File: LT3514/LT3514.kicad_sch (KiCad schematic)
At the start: 15 parts, among them U1 LT3514xUFD

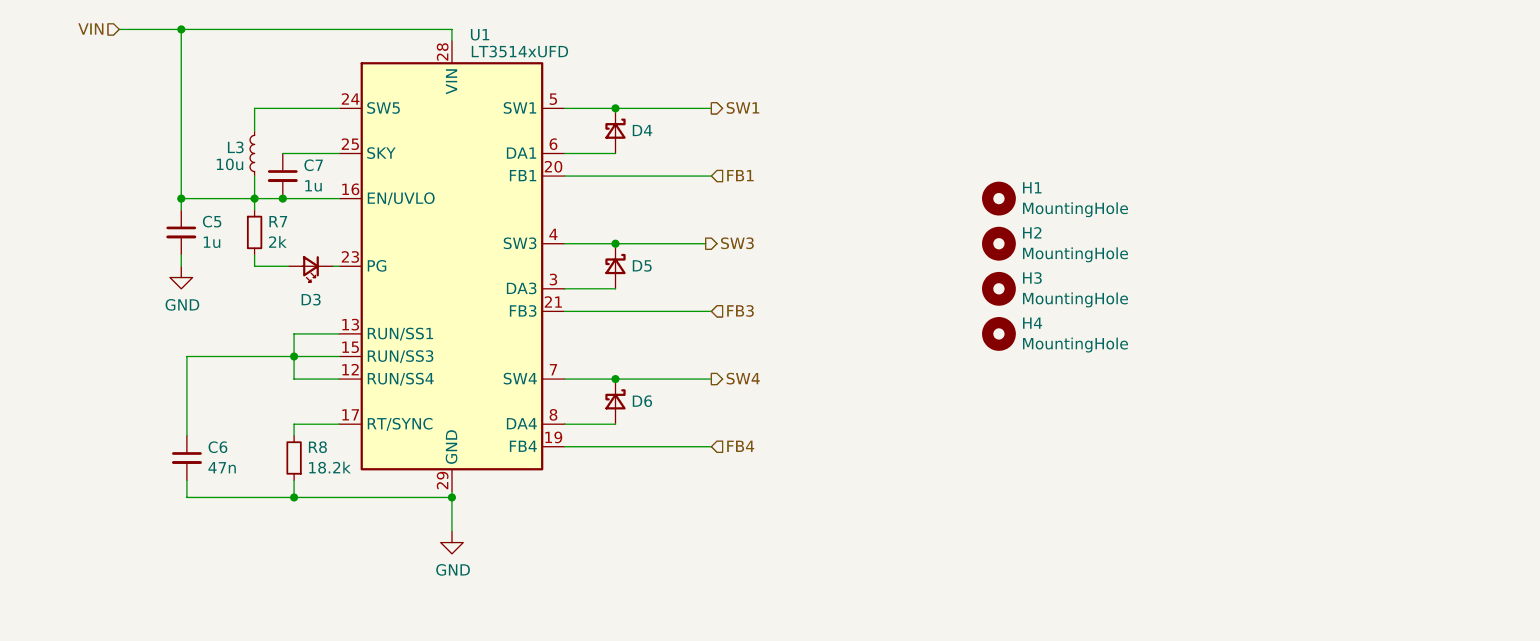
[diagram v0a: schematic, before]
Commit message: update files
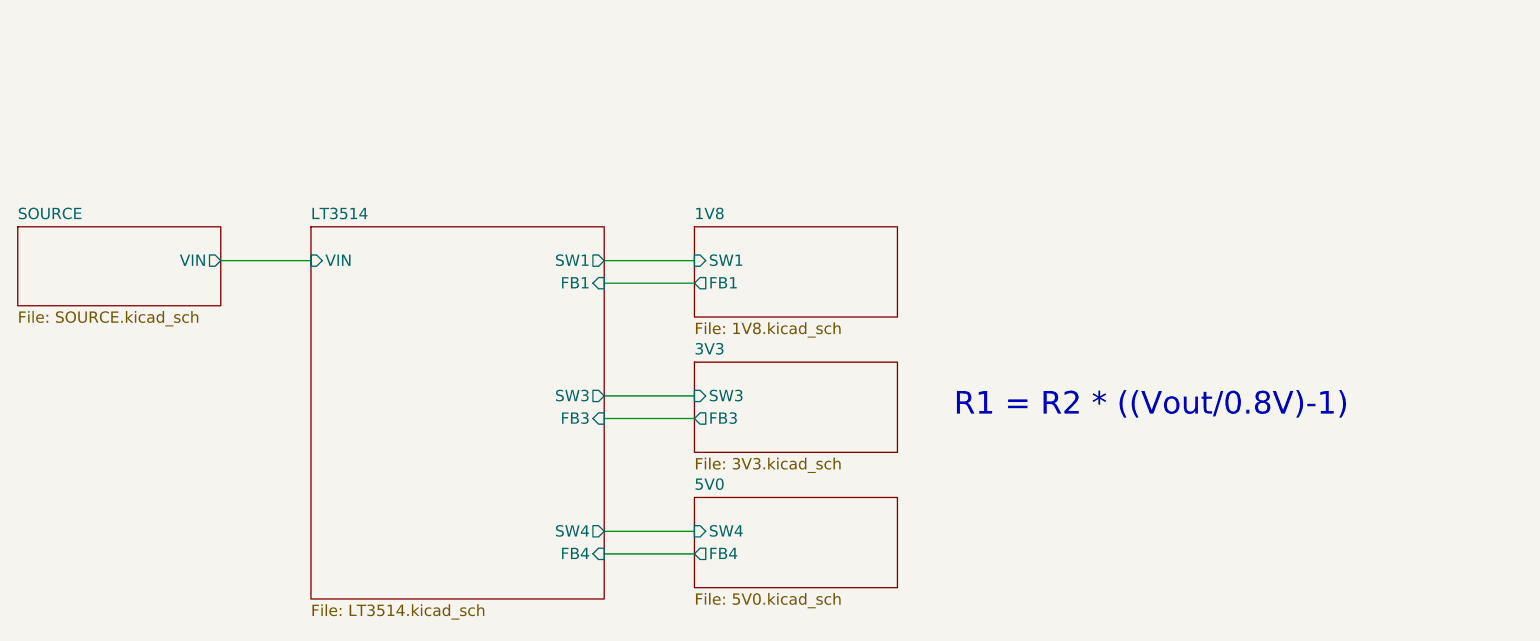
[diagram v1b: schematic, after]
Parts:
- removed C5, C7: 1u, Capacitor_SMD:C_0805_2012Metric, symbol Device:C_Small
- removed C6: 47n, Capacitor_SMD:C_0805_2012Metric, symbol Device:C_Small
- removed D3: LED_Small, LED_SMD:LED_0805_2012Metric, symbol Device:LED_Small
- removed D4, D5, D6: D_Schottky_Small, LT3514:B290, symbol Device:D_Schottky_Small
- removed H1, H2, H3, H4: MountingHole, MountingHole:MountingHole_3.2mm_M3_Pad_Via, symbol Mechanical:MountingHole
- removed L3: 10u, LT3514:EPL3015, symbol Device:L_Small
- removed R7: 2k, Resistor_SMD:R_0805_2012Metric, symbol Device:R_Small
- removed R8: 18.2k, Resistor_SMD:R_0805_2012Metric, symbol Device:R_Small
- removed U1: LT3514xUFD, Package_DFN_QFN:QFN-28-1EP_4x5mm_P0.5mm_EP2.65x3.65mm_ThermalVias, symbol Regulator_Switching:LT3514xUFD
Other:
- added sheet 1V8 (1V8.kicad_sch)
- added sheet 3V3 (3V3.kicad_sch)
- added sheet 5V0 (5V0.kicad_sch)
- added sheet LT3514 (LT3514.kicad_sch)
- added sheet SOURCE (SOURCE.kicad_sch)
- note added: "R1 = R2 * ((Vout/0.8V)-1)"
